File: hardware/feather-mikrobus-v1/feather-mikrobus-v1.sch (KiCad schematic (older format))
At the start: 22 parts, among them J1 Adafruit_Feather_socket_heade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, J2 Adafruit_Feather_socket_heade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, J3 mikroBUS_socket_header_left_p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, J4 mikroBUS_socket_header_right_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, SW1 FCD-000051, SW2 FCD-000049, SW3 FCD-000049

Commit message: [WIP] Update Adafruit Feather legacy footprints
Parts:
- J1: value Adafruit_Feather_socket_header_left_pth-Flying_Camp_Design -> FCD-000047; footprint Flying_Camp_Design:Adafruit_Feather_socket_header_left_pth -> Flying_Camp_Design:TE_6-534237-4; symbol feather-mikrobus-v1-rescue:Adafruit_Feather_socket_header_left_pth-Flying_Camp_Design -> Flying_Camp_Design:FCD-000047; Manufacturer TE Connectivity -> TE Connectivity AMP Connectors; Part Number (none) -> 6-534237-4; Vendor Digi-Key -> (none); Vendor Part Number A32549-ND -> (none); Vendor URL https://www.digikey.com/short/z8mb48 -> (none)
- J2: value Adafruit_Feather_socket_header_right_pth-Flying_Camp_Design -> FCD-000048; footprint Flying_Camp_Design:Adafruit_Feather_socket_header_right_pth -> Flying_Camp_Design:TE_6-534237-0; symbol feather-mikrobus-v1-rescue:Adafruit_Feather_socket_header_right_pth-Flying_Camp_Design -> Flying_Camp_Design:FCD-000048; Manufacturer TE Connectivity -> TE Connectivity AMP Connectors; Part Number (none) -> 6-534237-0; Vendor Digi-Key -> (none); Vendor Part Number A32911-ND -> (none); Vendor URL https://www.digikey.com/short/z8mbmc -> (none)
- J3: value mikroBUS_socket_header_left_pth-Flying_Camp_Design -> FCD-000050; footprint Flying_Camp_Design:mikroBUS_socket_header_left_pth -> Flying_Camp_Design:TE_5-534237-6; symbol feather-mikrobus-v1-rescue:mikroBUS_socket_header_left_pth-Flying_Camp_Design -> Flying_Camp_Design:FCD-000050; Manufacturer TE Connectivity -> TE Connectivity AMP Connectors; Part Number (none) -> 5-534237-6; Vendor Digi-Key -> (none); Vendor Part Number A32909-ND -> (none); Vendor URL https://www.digikey.com/short/z8mbmb -> (none)
- J4: value mikroBUS_socket_header_right_pth-Flying_Camp_Design -> FCD-000050; footprint Flying_Camp_Design:mikroBUS_socket_header_right_pth -> Flying_Camp_Design:TE_5-534237-6; symbol feather-mikrobus-v1-rescue:mikroBUS_socket_header_right_pth-Flying_Camp_Design -> Flying_Camp_Design:FCD-000050; Manufacturer TE Connectivity -> TE Connectivity AMP Connectors; Part Number (none) -> 5-534237-6; Vendor Digi-Key -> (none); Vendor Part Number A32909-ND -> (none); Vendor URL https://www.digikey.com/short/z8mbmb -> (none)
- MOD1: renamed from MH1; value Adafruit_Feather_socket_mounting_holes-Flying_Camp_Design -> MODULE_ADAFRUIT_FEATHER; footprint Flying_Camp_Design:Adafruit_Feather_socket_mounting_holes -> Flying_Camp_Design:MODULE_ADAFRUIT_FEATHER; symbol feather-mikrobus-v1-rescue:Adafruit_Feather_socket_mounting_holes-Flying_Camp_Design -> Flying_Camp_Design:MODULE_ADAFRUIT_FEATHER
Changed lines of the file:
@@
 $EndComp
 $Comp
-L feather-mikrobus-v1-rescue:Adafruit_Feather_socket_mounting_holes-Flying_Camp_Design MH1
+L Flying_Camp_Design:MODULE_ADAFRUIT_FEATHER MOD1
 U 1 1 5E3B84FB
-P 5600 1700
-F 0 "MH1" H 5600 1800 50  0001 C CNN
-F 1 "Adafruit_Feather_socket_mounting_holes-Flying_Camp_Design" H 5600 1400 50  0001 C CNN
-F 2 "Flying_Camp_Design:Adafruit_Feather_socket_mounting_holes" H 5600 1300 50  0001 C CNN
-F 3 "" H 5600 1200 50  0001 C CNN
-	1    5600 1700
+P 5700 1600
+F 0 "MOD1" H 5700 1700 50  0001 C CNN
+F 1 "MODULE_ADAFRUIT_FEATHER" H 5700 1300 50  0001 C CNN
+F 2 "Flying_Camp_Design:MODULE_ADAFRUIT_FEATHER" H 5700 1200 50  0001 C CNN
+F 3 "https://learn.adafruit.com/adafruit-feather/feather-specification" H 5700 1100 50  0001 C CNN
+	1    5700 1600
 	1    0    0    -1
 $EndComp
 $Comp
-L feather-mikrobus-v1-rescue:Adafruit_Feather_socket_header_left_pth-Flying_Camp_Design J1
+L Flying_Camp_Design:FCD-000047 J1
 U 1 1 5E3B727D
-P 5200 2300
-F 0 "J1" H 5000 1300 50  0000 L CNN
-F 1 "Adafruit_Feather_socket_header_left_pth-Flying_Camp_Design" H 5200 1100 50  0001 C CNN
-F 2 "Flying_Camp_Design:Adafruit_Feather_socket_header_left_pth" H 5200 1000 50  0001 C CNN
-F 3 "" H 5200 900 50  0001 C CNN
-F 4 "TE Connectivity" H 5200 1300 50  0000 C CNN "Manufacturer"
-F 5 "6-534237-4" H 5200 1200 50  0000 C CNN "Manufacturer Part Number"
-F 6 "Digi-Key" H 5200 800 50  0001 C CNN "Vendor"
-F 7 "A32549-ND" H 5200 700 50  0001 C CNN "Vendor Part Number"
-F 8 "https://www.digikey.com/short/z8mb48" H 5200 600 50  0001 C CNN "Vendor URL"
-	1    5200 2300
+P 5100 2300
+F 0 "J1" H 4900 1300 50  0000 L CNN
+F 1 "FCD-000047" H 5100 1300 50  0000 C CNN
+F 2 "Flying_Camp_Design:TE_6-534237-4" H 5100 900 50  0001 C CNN
+F 3 "http://127.0.0.1:8000/part/FCD-000047/" H 5100 800 50  0001 C CNN
+F 4 "TE Connectivity AMP Connectors" H 5100 1100 50  0001 C CNN "Manufacturer"
+F 5 "6-534237-4" H 5100 1000 50  0001 C CNN "Manufacturer Part Number"
+F 6 "6-534237-4" H 5100 1200 50  0000 C CNN "Part Number"
+	1    5100 2300
 	1    0    0    -1
 $EndComp
 $Comp
-L feather-mikrobus-v1-rescue:Adafruit_Feather_socket_header_right_pth-Flying_Camp_Design J2
+L Flying_Camp_Design:FCD-000048 J2
 U 1 1 5E3B67CD
-P 5600 2500
-F 0 "J2" H 5000 1600 50  0000 L CNN
-F 1 "Adafruit_Feather_socket_header_right_pth-Flying_Camp_Design" H 5600 1500 50  0001 C CNN
-F 2 "Flying_Camp_Design:Adafruit_Feather_socket_header_right_pth" H 5600 1400 50  0001 C CNN
-F 3 "" H 5600 1300 50  0001 C CNN
-F 4 "TE Connectivity" H 5600 1700 50  0000 C CNN "Manufacturer"
-F 5 "6-534237-0" H 5600 1600 50  0000 C CNN "Manufacturer Part Number"
-F 6 "Digi-Key" H 5600 1200 50  0001 C CNN "Vendor"
-F 7 "A32911-ND" H 5600 1100 50  0001 C CNN "Vendor Part Number"
-F 8 "https://www.digikey.com/short/z8mbmc" H 5600 1000 50  0001 C CNN "Vendor URL"
-	1    5600 2500
-	1    0    0    -1
+P 5700 2500
+F 0 "J2" H 5100 1600 50  0000 L CNN
+F 1 "FCD-000048" H 5700 1700 50  0000 C CNN
+F 2 "Flying_Camp_Design:TE_6-534237-0" H 5700 1300 50  0001 C CNN
+F 3 "http://127.0.0.1:8000/part/FCD-000048/" H 5700 1200 50  0001 C CNN
+F 4 "TE Connectivity AMP Connectors" H 5700 1500 50  0001 C CNN "Manufacturer"
+F 5 "6-534237-0" H 5700 1400 50  0001 C CNN "Manufacturer Part Number"
+F 6 "6-534237-0" H 5700 1600 50  0000 C CNN "Part Number"
+	1    5700 2500
+	-1   0    0    -1
 $EndComp
 $Comp
@@
 $EndComp
 $Comp
-L feather-mikrobus-v1-rescue:mikroBUS_socket_header_left_pth-Flying_Camp_Design J3
+L Flying_Camp_Design:FCD-000050 J3
 U 1 1 5E3C6EE3
-P 2500 5000
-F 0 "J3" H 2300 4400 50  0000 L CNN
-F 1 "mikroBUS_socket_header_left_pth-Flying_Camp_Design" H 2500 4200 50  0001 C CNN
-F 2 "Flying_Camp_Design:mikroBUS_socket_header_left_pth" H 2500 4100 50  0001 C CNN
-F 3 "" H 2500 4000 50  0001 C CNN
-F 4 "TE Connectivity" H 2500 4400 50  0000 C CNN "Manufacturer"
-F 5 "5-534237-6" H 2500 4300 50  0000 C CNN "Manufacturer Part Number"
-F 6 "Digi-Key" H 2500 3900 50  0001 C CNN "Vendor"
-F 7 "A32909-ND" H 2500 3800 50  0001 C CNN "Vendor Part Number"
-F 8 "https://www.digikey.com/short/z8mbmb" H 2500 3700 50  0001 C CNN "Vendor URL"
-	1    2500 5000
+P 2400 5000
+F 0 "J3" H 2200 4400 50  0000 L CNN
+F 1 "FCD-000050" H 2400 4400 50  0000 C CNN
+F 2 "Flying_Camp_Design:TE_5-534237-6" H 2400 4000 50  0001 C CNN
+F 3 "http://127.0.0.1:8000/part/FCD-000050/" H 2400 3900 50  0001 C CNN
+F 4 "TE Connectivity AMP Connectors" H 2400 4200 50  0001 C CNN "Manufacturer"
+F 5 "5-534237-6" H 2400 4100 50  0001 C CNN "Manufacturer Part Number"
+F 6 "5-534237-6" H 2400 4300 50  0000 C CNN "Part Number"
+	1    2400 5000
 	1    0    0    -1
 $EndComp
 $Comp
-L feather-mikrobus-v1-rescue:mikroBUS_socket_header_right_pth-Flying_Camp_Design J4
+L Flying_Camp_Design:FCD-000050 J4
 U 1 1 5E3C7996
-P 2900 5000
-F 0 "J4" H 2300 4300 50  0000 L CNN
-F 1 "mikroBUS_socket_header_right_pth-Flying_Camp_Design" H 2900 4200 50  0001 C CNN
-F 2 "Flying_Camp_Design:mikroBUS_socket_header_right_pth" H 2900 4100 50  0001 C CNN
-F 3 "" H 2900 4000 50  0001 C CNN
-F 4 "TE Connectivity" H 2900 4400 50  0000 C CNN "Manufacturer"
-F 5 "5-534237-6" H 2900 4300 50  0000 C CNN "Manufacturer Part Number"
-F 6 "Digi-Key" H 2900 3900 50  0001 C CNN "Vendor"
-F 7 "A32909-ND" H 2900 3800 50  0001 C CNN "Vendor Part Number"
-F 8 "https://www.digikey.com/short/z8mbmb" H 2900 3700 50  0001 C CNN "Vendor URL"
-	1    2900 5000
-	1    0    0    -1
+P 3000 5000
+F 0 "J4" H 2400 4300 50  0000 L CNN
+F 1 "FCD-000050" H 3000 4400 50  0000 C CNN
+F 2 "Flying_Camp_Design:TE_5-534237-6" H 3000 4000 50  0001 C CNN
+F 3 "http://127.0.0.1:8000/part/FCD-000050/" H 3000 3900 50  0001 C CNN
+F 4 "TE Connectivity AMP Connectors" H 3000 4200 50  0001 C CNN "Manufacturer"
+F 5 "5-534237-6" H 3000 4100 50  0001 C CNN "Manufacturer Part Number"
+F 6 "5-534237-6" H 3000 4300 50  0000 C CNN "Part Number"
+	1    3000 5000
+	-1   0    0    -1
 $EndComp
 $Comp

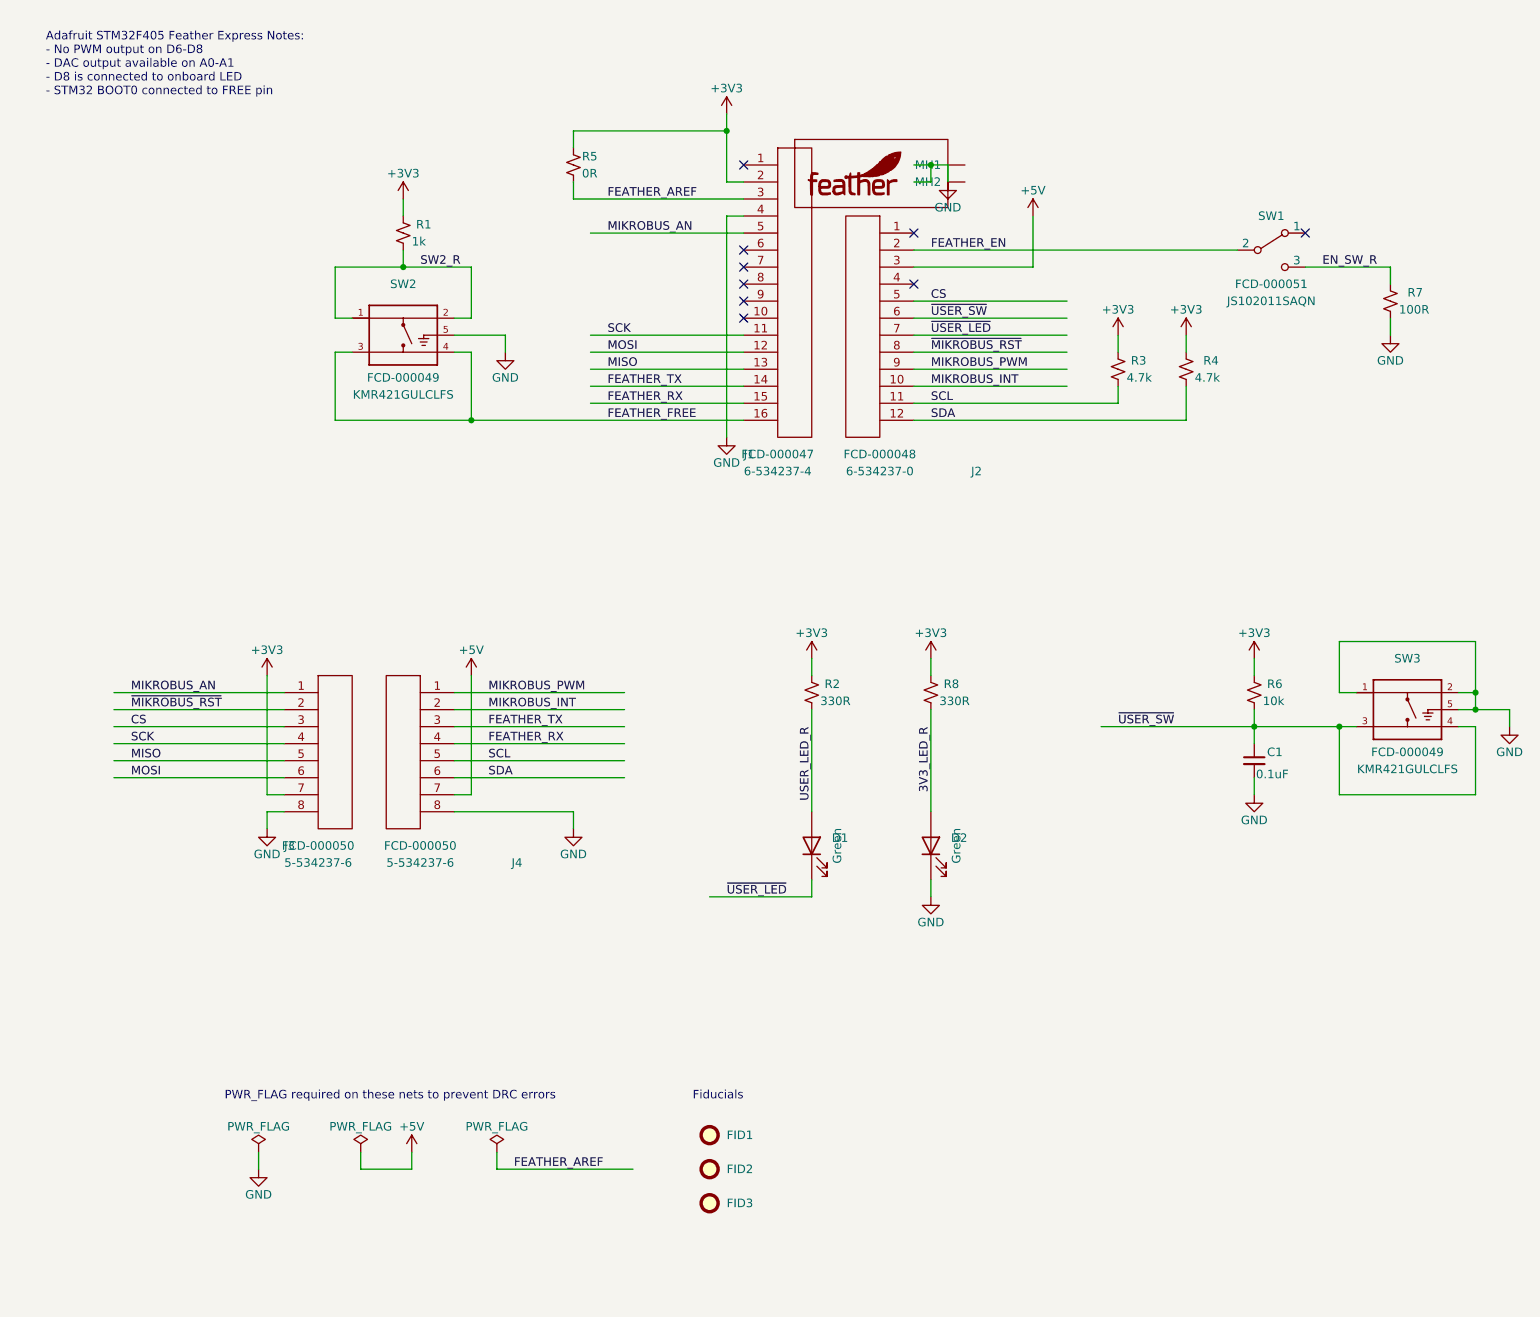
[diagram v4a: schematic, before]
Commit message: [WIP] Update legacy mikroBUS symbols
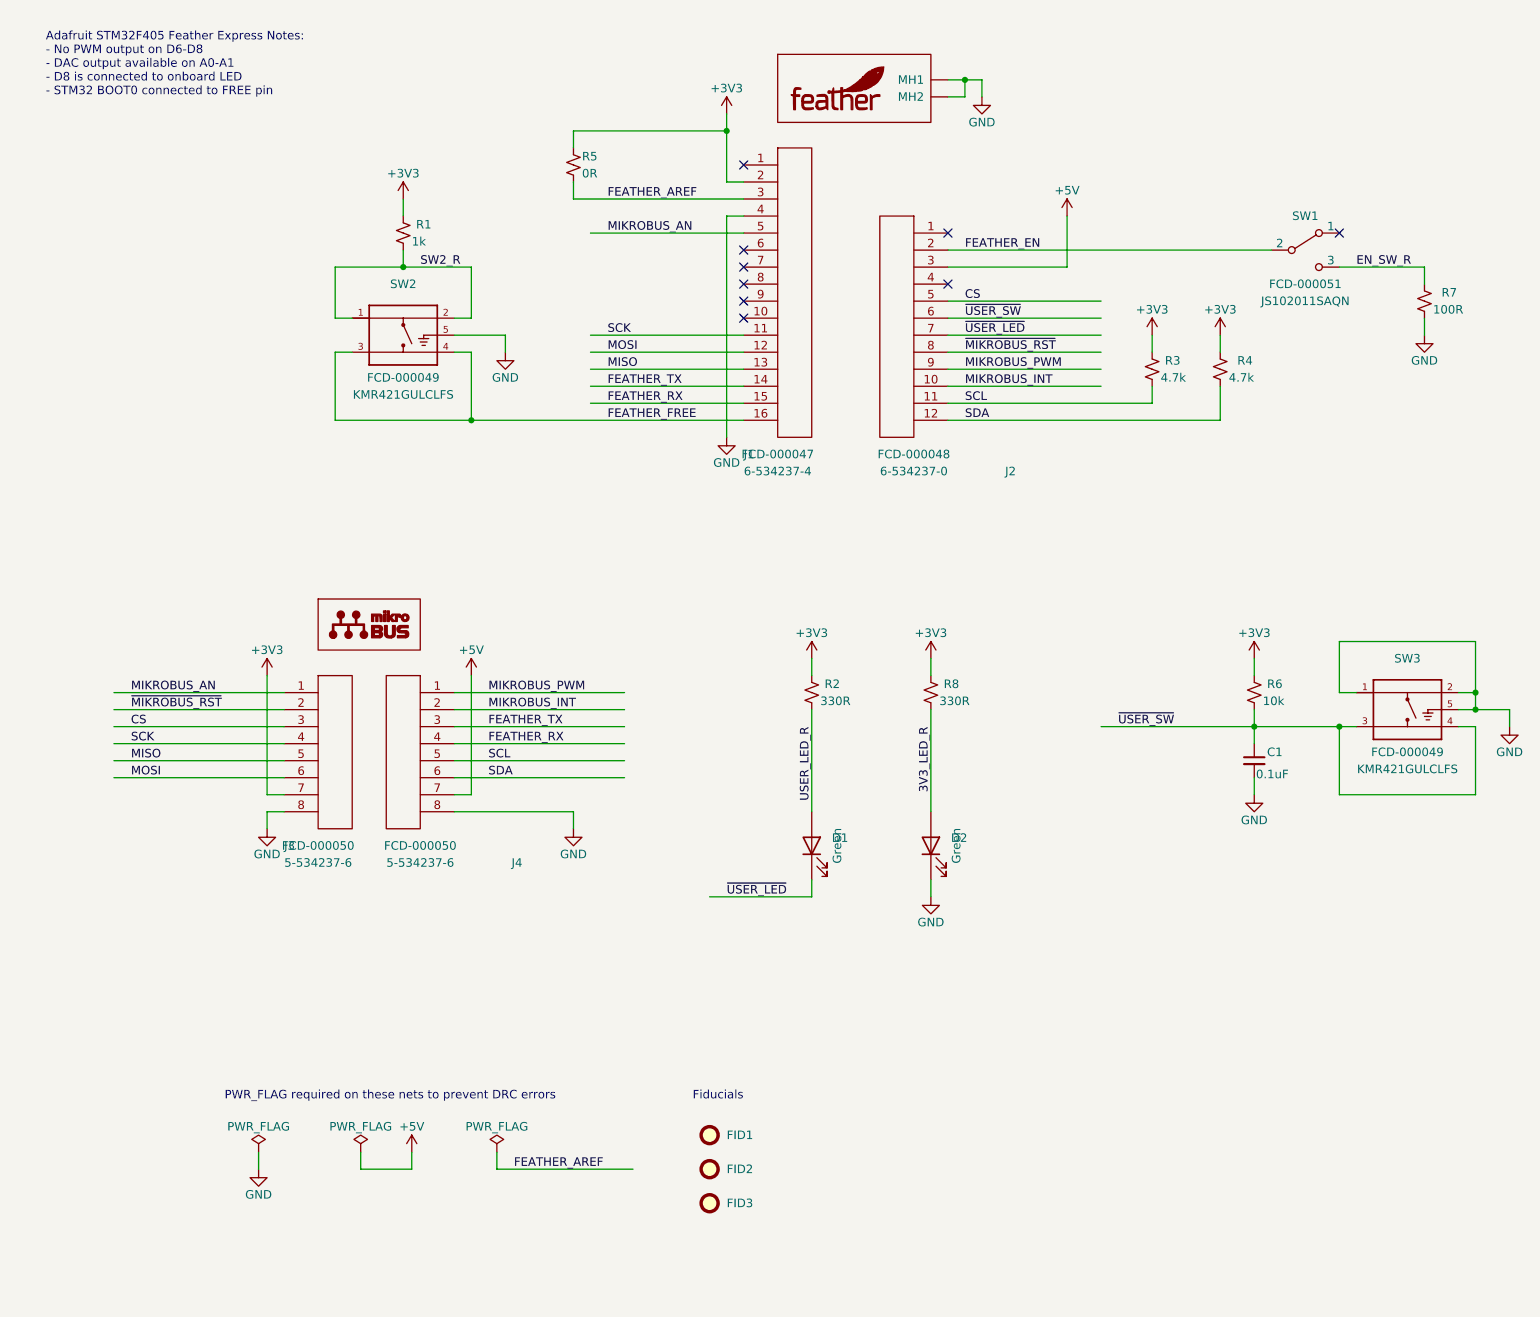
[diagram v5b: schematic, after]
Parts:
- added MOD2: MODULE_MIKROBUS, Flying_Camp_Design:MODULE_MIKROBUS, symbol Flying_Camp_Design:MODULE_MIKROBUS
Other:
- moved on the sheet: J2, R3, R4, R7, SW1
